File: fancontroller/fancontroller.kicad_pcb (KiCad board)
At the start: 2 copper layers, 98.2 x 84.4 mm, 84 parts, among them J1 Power, J2 Debug, M1 FAN0, M2 FAN0, M3 FAN0, M4 FAN0, M5 FAN0, M6 FAN0, P1 USB_C_Plug_USB2.0, Q1 SS8050-G, Q10 AO3401A, Q11 AO3400A, Q12 AO3401A, Q13 AO3400A, Q14 AO3401A, Q2 SS8050-G, Q3 AO3400A, Q4 AO3401A, Q5 AO3400A, Q6 AO3401A, Q7 AO3400A, Q8 AO3401A, Q9 AO3400A, SW1 Reset, U1 ESP32-WROOM-32, U2 CH340C, U3 BD9D300MUV, U4 AMS1117-3.3

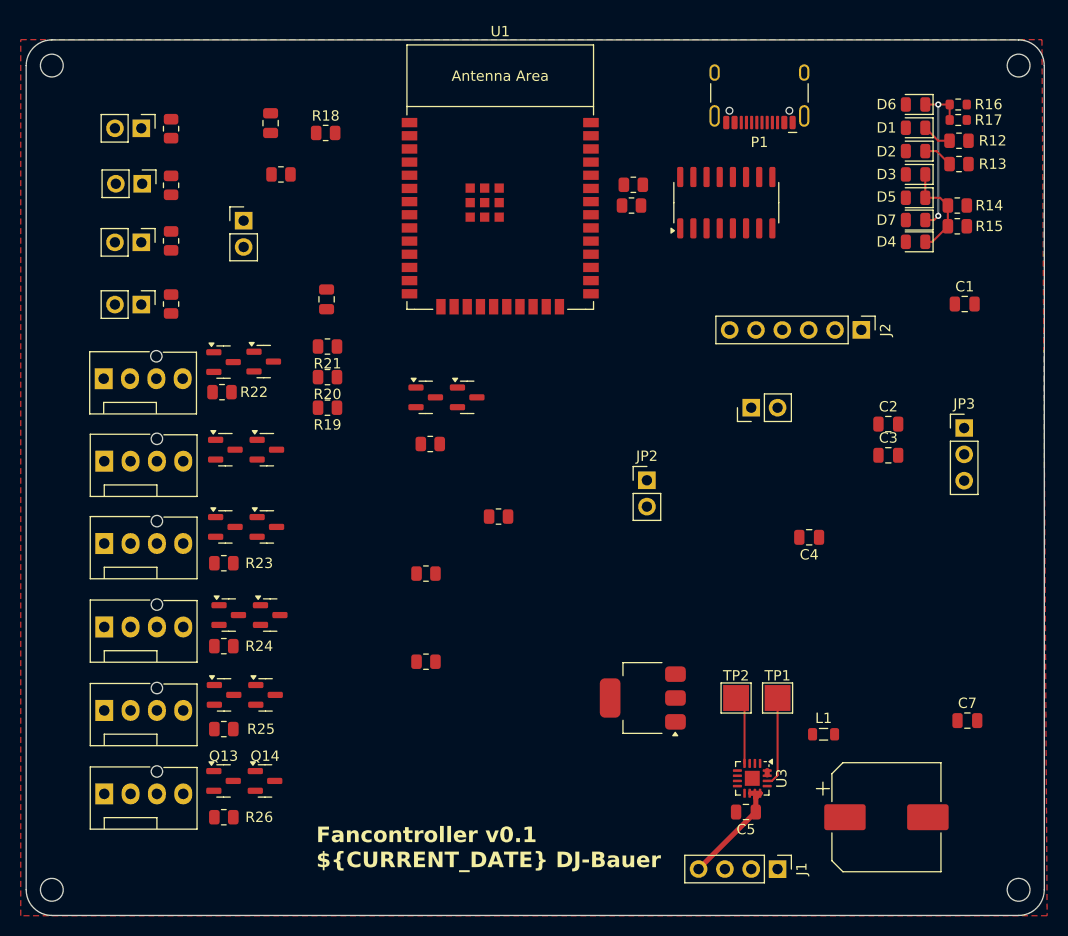
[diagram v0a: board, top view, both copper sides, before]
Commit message: edit schematic
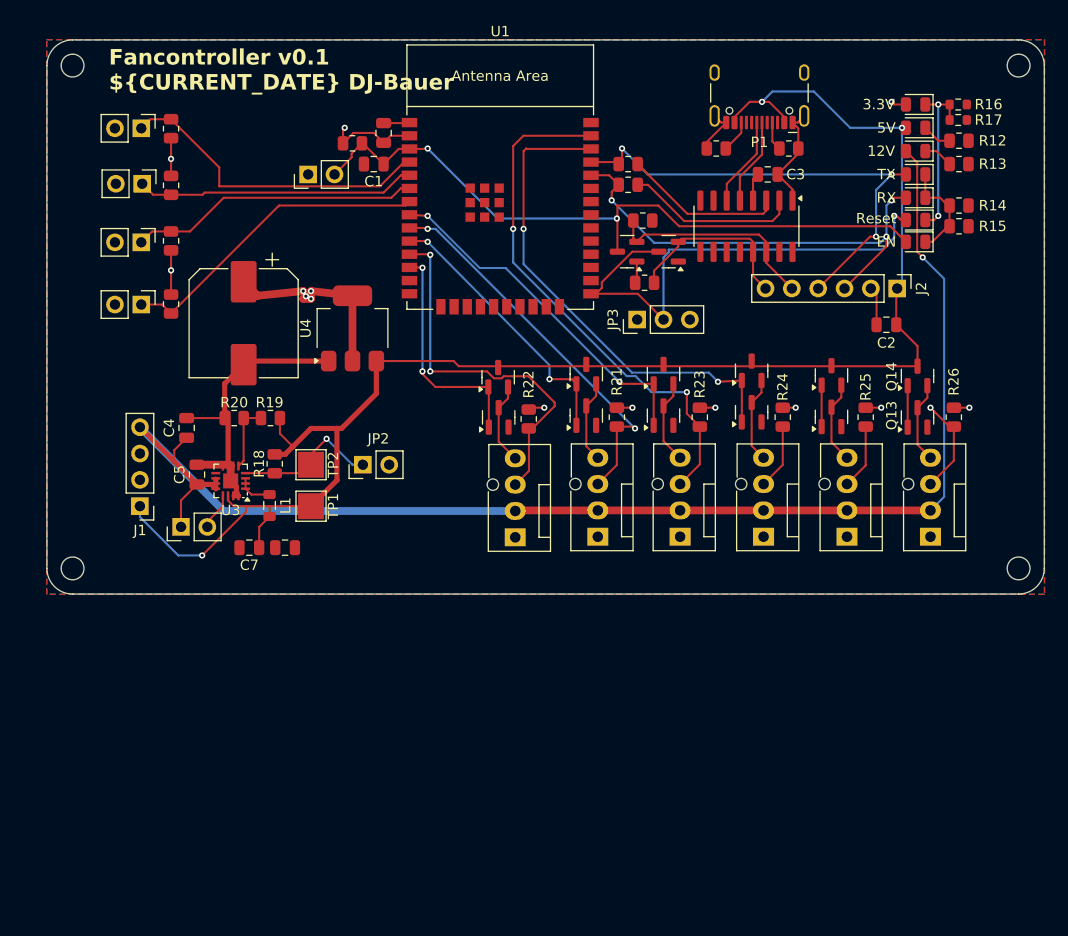
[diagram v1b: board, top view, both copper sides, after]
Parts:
- U3: footprint Package_DFN_QFN:VQFN-16-1EP_3x3mm_P0.5mm_EP1.45x1.45mm -> DJCustom:VQFN-16-1EP_3x3mm_P0.5mm_EP1.45x1.45mm
- U4: footprint Package_TO_SOT_SMD:SOT-223-3_TabPin2 -> Package_TO_SOT_SMD:SOT-223
- moved M6 83.5 mm to (113.8, 134.4), turned to 90 degrees
- moved R26 80.3 mm to (116.0, 122.9), turned to -90 degrees
- moved C8 78.2 mm to (47.5, 113.8), turned to -90 degrees
- moved Q13 75.6 mm to (112.5, 122.9), turned to 90 degrees
- moved Q14 74.1 mm to (112.5, 118.9), turned to 90 degrees
- moved M5 73.6 mm to (105.7, 134.4), turned to 90 degrees
- moved C7 71.2 mm to (48.0, 135.5), turned to 180 degrees
- moved J1 70.8 mm to (37.5, 131.5), turned to 180 degrees
- moved R25 68.8 mm to (107.5, 122.9), turned to -90 degrees
- moved Q11 64.4 mm to (104.2, 122.9), turned to 90 degrees
- moved M4 64.2 mm to (97.7, 134.4), turned to 90 degrees
- moved Q12 62.7 mm to (104.2, 118.9), turned to 90 degrees
- moved C5 62.2 mm to (43.0, 128.4), turned to 90 degrees
- moved C4 61.0 mm to (42.0, 124.0), turned to 90 degrees
- moved C1 58.6 mm to (60.0, 98.5), turned to 180 degrees
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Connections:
- U1 pad 11: /Tacho 1 -> /Tacho 0
- U1 pad 12: /PWM 2 -> /PWM 0
- U1 pad 27: /Tacho 2 -> /PWM 5
- U1 pad 28: /PWM 3 -> /Tacho 5
- U1 pad 36: /PWM 5 -> /PWM 3
- U1 pad 37: /Tacho 5 -> /Tacho 2
- U1 pad 8: /PWM 0 -> /PWM 2
- U1 pad 9: /Tacho 0 -> /Tacho 1
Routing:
- net +5V: track 8.68 -> 154.3 mm, vias 0 -> 3
- net +12V: track 10.7 -> 134.6 mm, vias 0 -> 1
- net EN: track 0.00 -> 66.8 mm, vias 0 -> 2
- net /Tacho 2: track 0.00 -> 51.3 mm, vias 0 -> 2
- net GND: track 0.43 -> 51.5 mm
- net RST: track 0.00 -> 49.2 mm, vias 0 -> 1
- net /PWM 3: track 0.00 -> 47.5 mm, vias 0 -> 2
- net +3.3V: track 0.00 -> 47.3 mm, vias 0 -> 14
- net TX: track 0.00 -> 47.1 mm, vias 0 -> 3
- net RX: track 0.00 -> 45.1 mm, vias 0 -> 3
- net /Tacho 1: track 0.00 -> 37.9 mm, vias 0 -> 2
- net /Tacho 0: track 0.00 -> 36.4 mm, vias 0 -> 2
- net /PWM 2: track 0.00 -> 34.4 mm, vias 0 -> 2
- net TMP3: track 0.00 -> 31.3 mm
- net TMP0: track 0.00 -> 30.7 mm
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- added copper zone on B.Cu, net +3.3V
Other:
- board size 98.2 x 84.4 mm -> 96.2 x 53.4 mm
